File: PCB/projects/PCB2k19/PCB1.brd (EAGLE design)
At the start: 190.7 x 218 mm, 223 parts, among them Q1M1 AOD482, Q1M2 AOD482, Q1M3 AOD482, Q1M4 AOD482, U1M1 VNH5019, U1M2 VNH5019, U1M3 VNH5019, U1M4 VNH5019

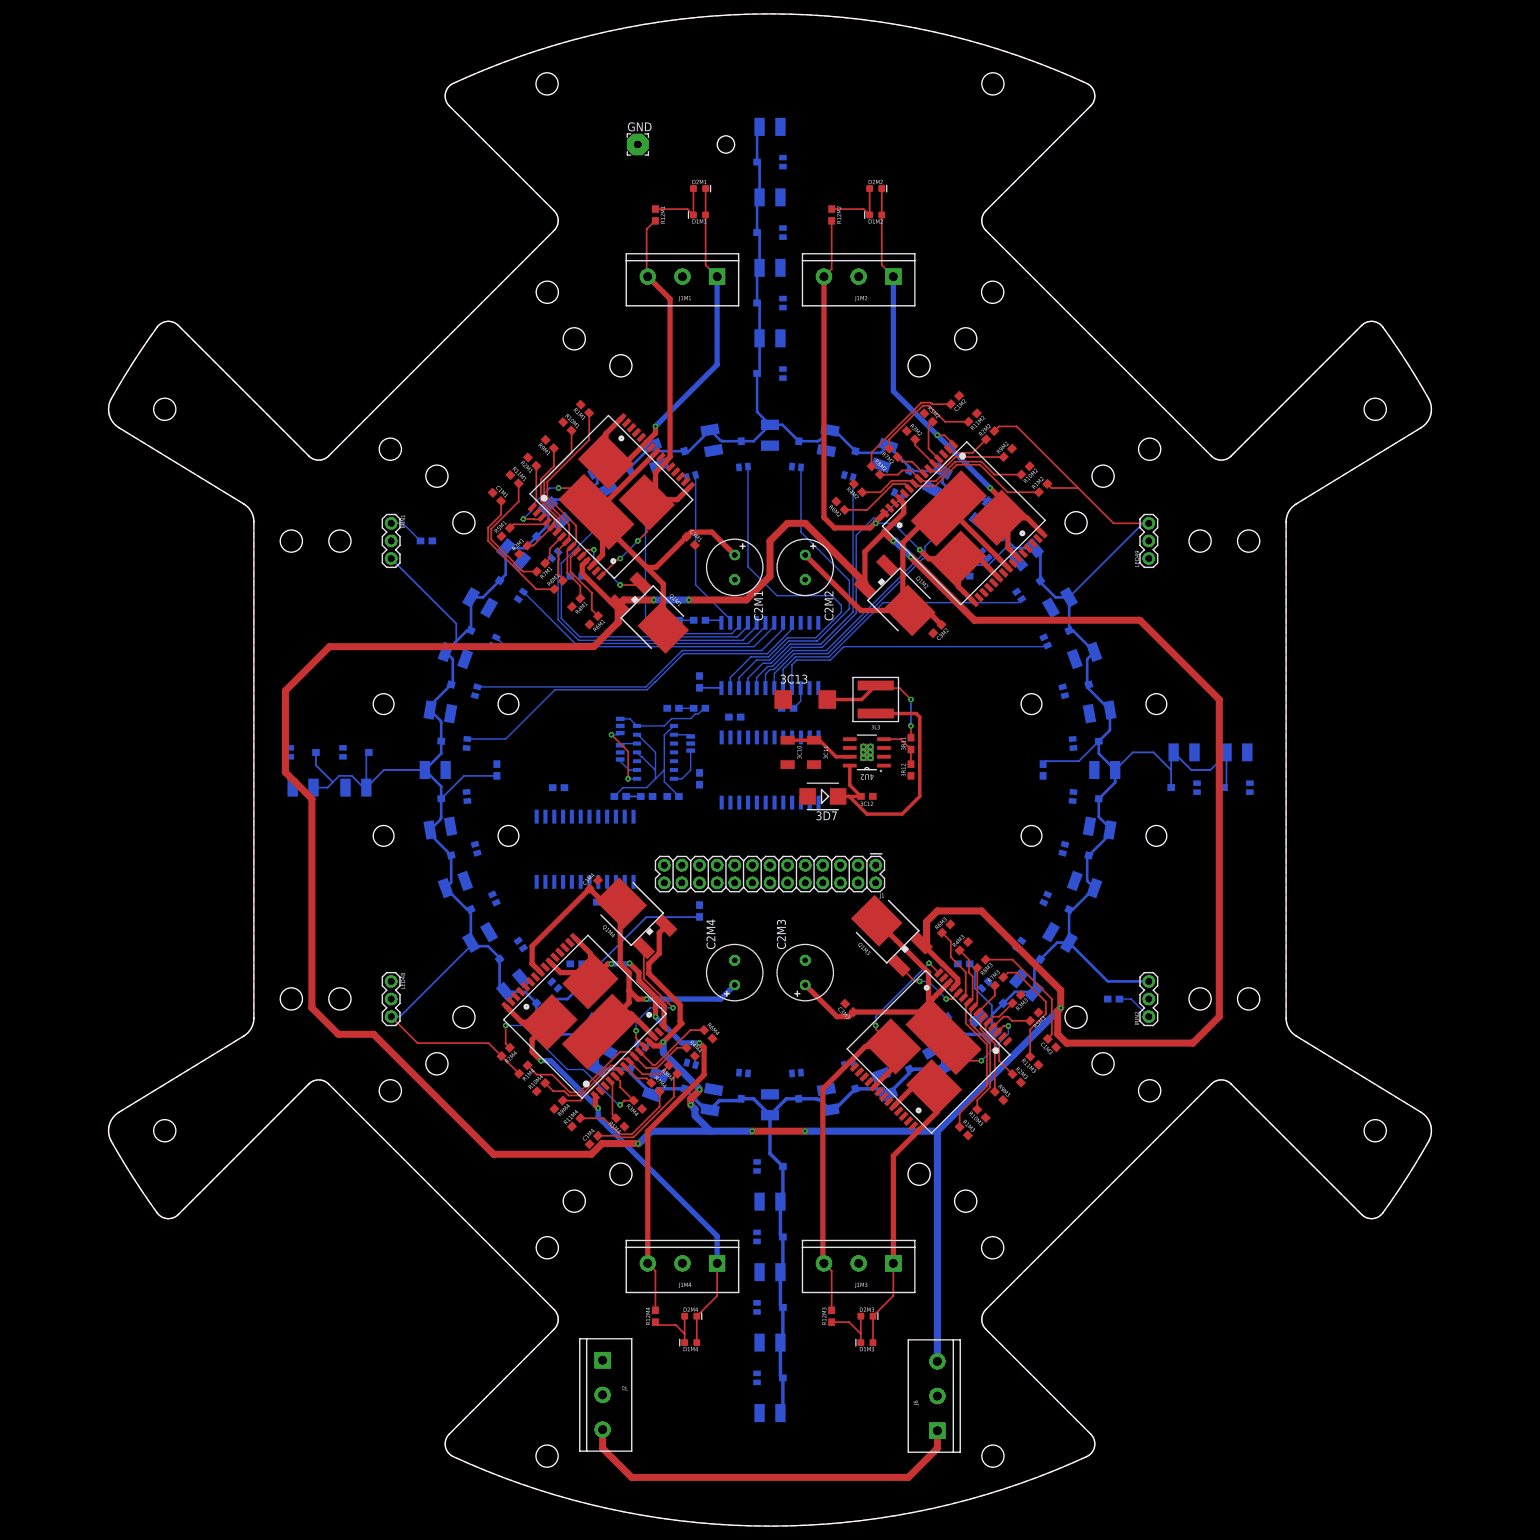
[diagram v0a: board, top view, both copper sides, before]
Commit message: 19/3 Finally finished PCB everything gerber in here too bye maybe make a 3d model sometime when im free
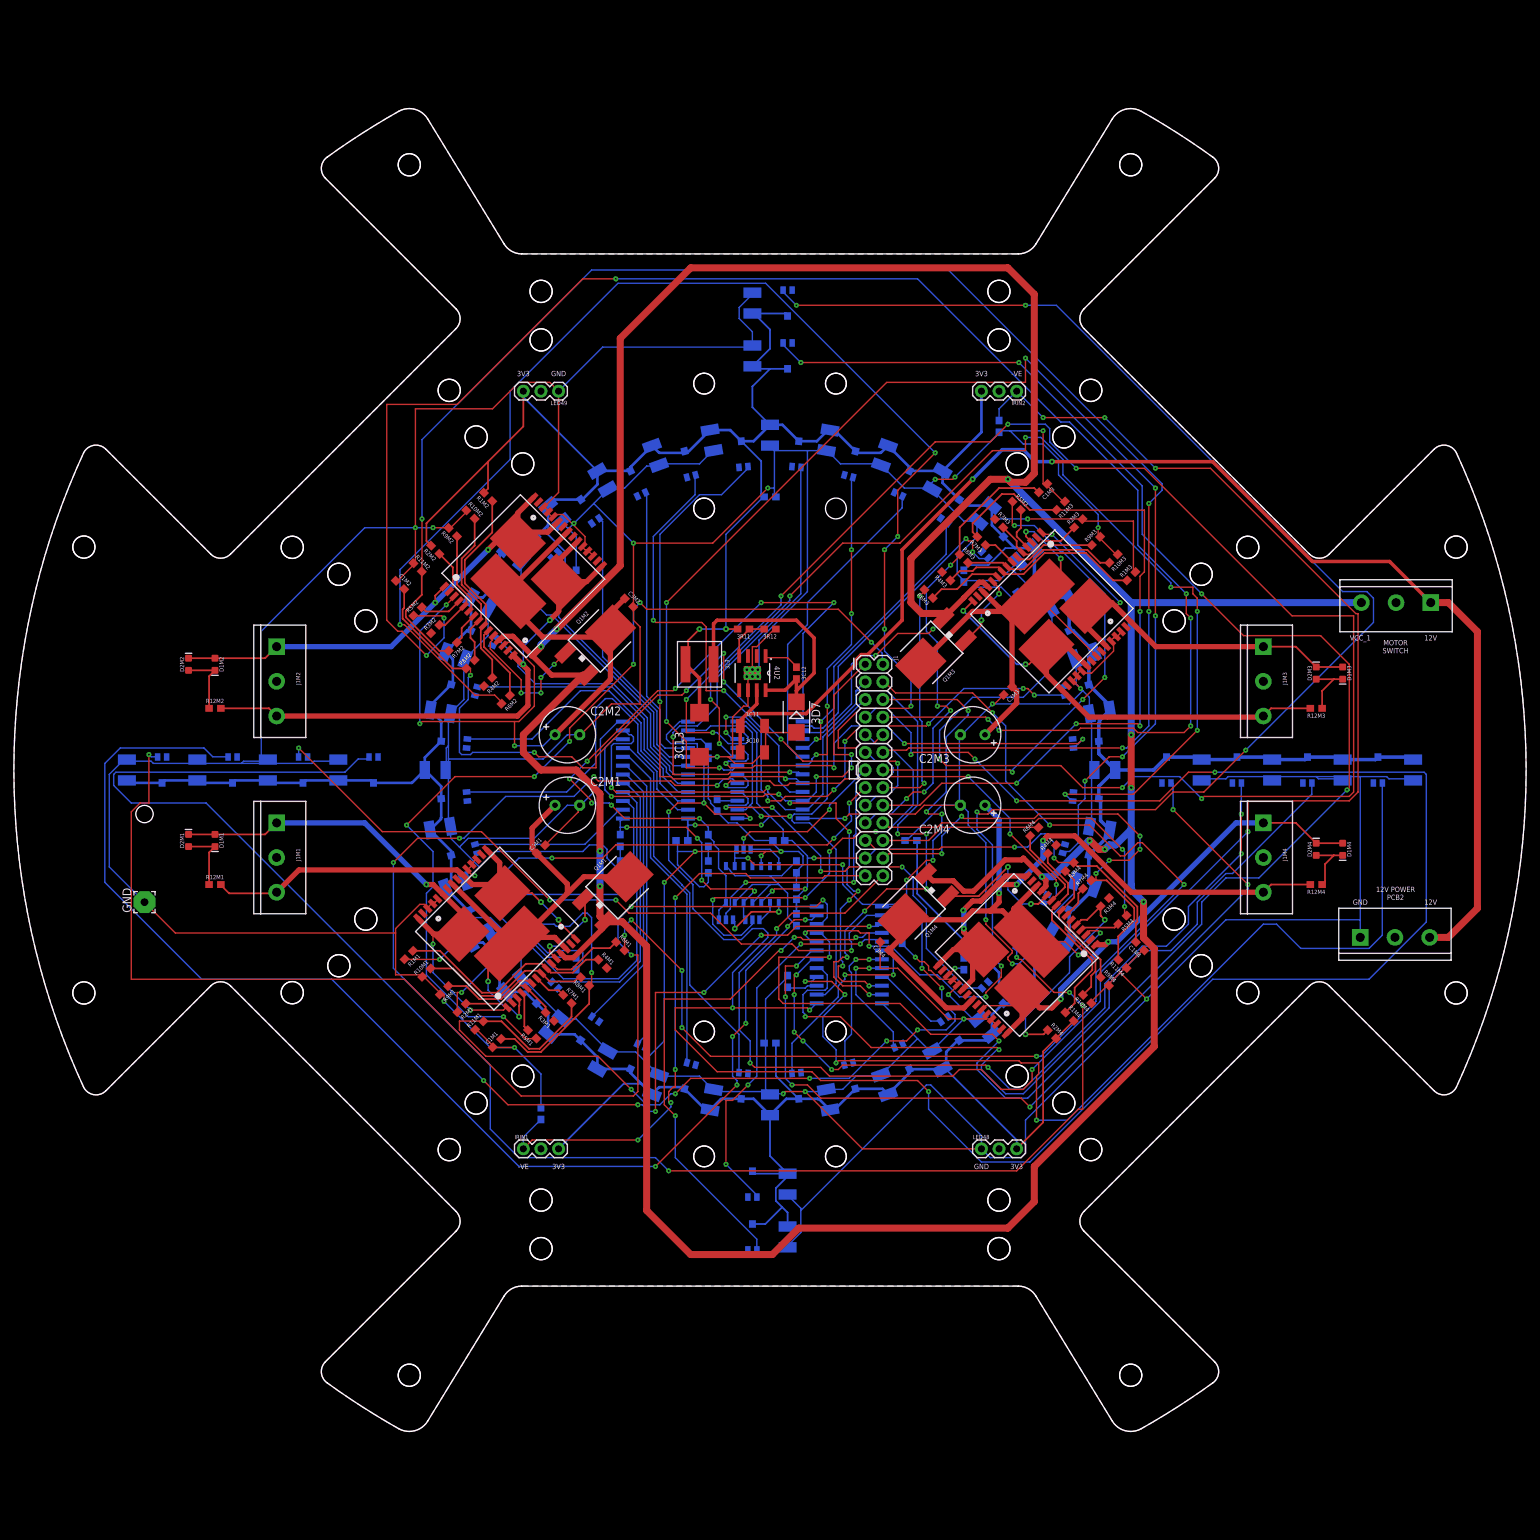
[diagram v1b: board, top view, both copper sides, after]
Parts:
- moved J6 139.0 mm to (95.2, 24.1), turned to 180 degrees
- moved LED41 131.1 mm to (-92.7, 0.00), turned to 90 degrees
- moved LED47 131.1 mm to (92.7, 0.00), turned to 270 degrees
- moved GND 130.3 mm to (-90.2, -19.1), turned to 90 degrees
- moved J2 125.1 mm to (85.1, -24.1), turned to 0 degrees
- moved PT41 123.9 mm to (-87.6, 0.00), turned to 270 degrees
- moved PT47 123.9 mm to (87.6, 0.00), turned to 90 degrees
- moved D2M2 120.5 mm to (-83.8, 15.2), turned to 90 degrees
- moved D2M1 119.4 mm to (-83.8, -10.2), turned to 90 degrees
- moved D1M3 118.4 mm to (82.5, 14.0), turned to 270 degrees
- moved D1M4 117.9 mm to (82.5, -11.4), turned to 270 degrees
- moved LED40 116.7 mm to (-82.5, 0.00), turned to 90 degrees
- moved LED46 116.7 mm to (82.5, 0.00), turned to 270 degrees
- moved R12M1 115.5 mm to (-80.0, -16.5), turned to 0 degrees
- moved D1M2 115.2 mm to (-80.0, 15.2), turned to 270 degrees
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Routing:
- net GND: track 0.00 -> 1439.5 mm, vias 0 -> 29
- net S3: track 0.00 -> 343.4 mm, vias 0 -> 10
- net INAM2: track 0.00 -> 261.4 mm, vias 0 -> 8
- net N$77: track 0.00 -> 259.2 mm, vias 0 -> 8
- net N$97: track 0.00 -> 256.4 mm, vias 0 -> 6
- net GATE2: track 5.28 -> 247.9 mm, vias 0 -> 7
- net N$98: track 0.00 -> 238.5 mm, vias 0 -> 8
- net PWMM2: track 15.7 -> 239.9 mm, vias 0 -> 4
- net N$83: track 0.00 -> 220.3 mm, vias 0 -> 8
- net INBM2: track 0.00 -> 200.4 mm, vias 0 -> 6
- net N$93: track 0.00 -> 190.9 mm, vias 0 -> 6
- net N$81: track 0.00 -> 187.5 mm, vias 0 -> 8
- net N$95: track 0.00 -> 180.6 mm, vias 0 -> 6
- net N$96: track 0.00 -> 177.8 mm, vias 0 -> 4
- net INBM1: track 0.00 -> 171.9 mm, vias 0 -> 8
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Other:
- board size 190.7 x 218 mm -> 218 x 190.7 mm
- board text added: "-VE"
- board text added: "12V"
- board text added: "12V POWER PCB2"
- board text added: "3V3"
- board text added: "GND"
- board text added: "MOTOR SWITCH"
- board text added: "VCC_1"
